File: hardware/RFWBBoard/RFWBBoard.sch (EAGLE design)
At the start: 123 parts, among them IC1 24LC025ST, J1 CON-71742-3003-BOT, M1 MOUNT-HOLE3.3, M2 MOUNT-HOLE3.3, M3 MOUNT-HOLE3.3, M4 MOUNT-HOLE3.3, M5 FIDUCIAL1X2, M6 FIDUCIAL1X2, M7 FIDUCIAL1X2, M8 FIDUCIAL1X2, U1 MAX2830IPC-7351, U2 LDB212G4010C-001, U3 LDB212G4010C-001, U4 AD8132MSOP8, U5 AD8132MSOP8, U6 AD8132MSOP8, U7 AD8132MSOP8, U8 ICS83021I, U9 ICS85320I, X1 SMA-SMD, X2 SMA-SMD, X3 FOX924B, X4 SMA-SMD, X5 SMA-SMD, X6 SMA-SMD, X7 SMA-SMD

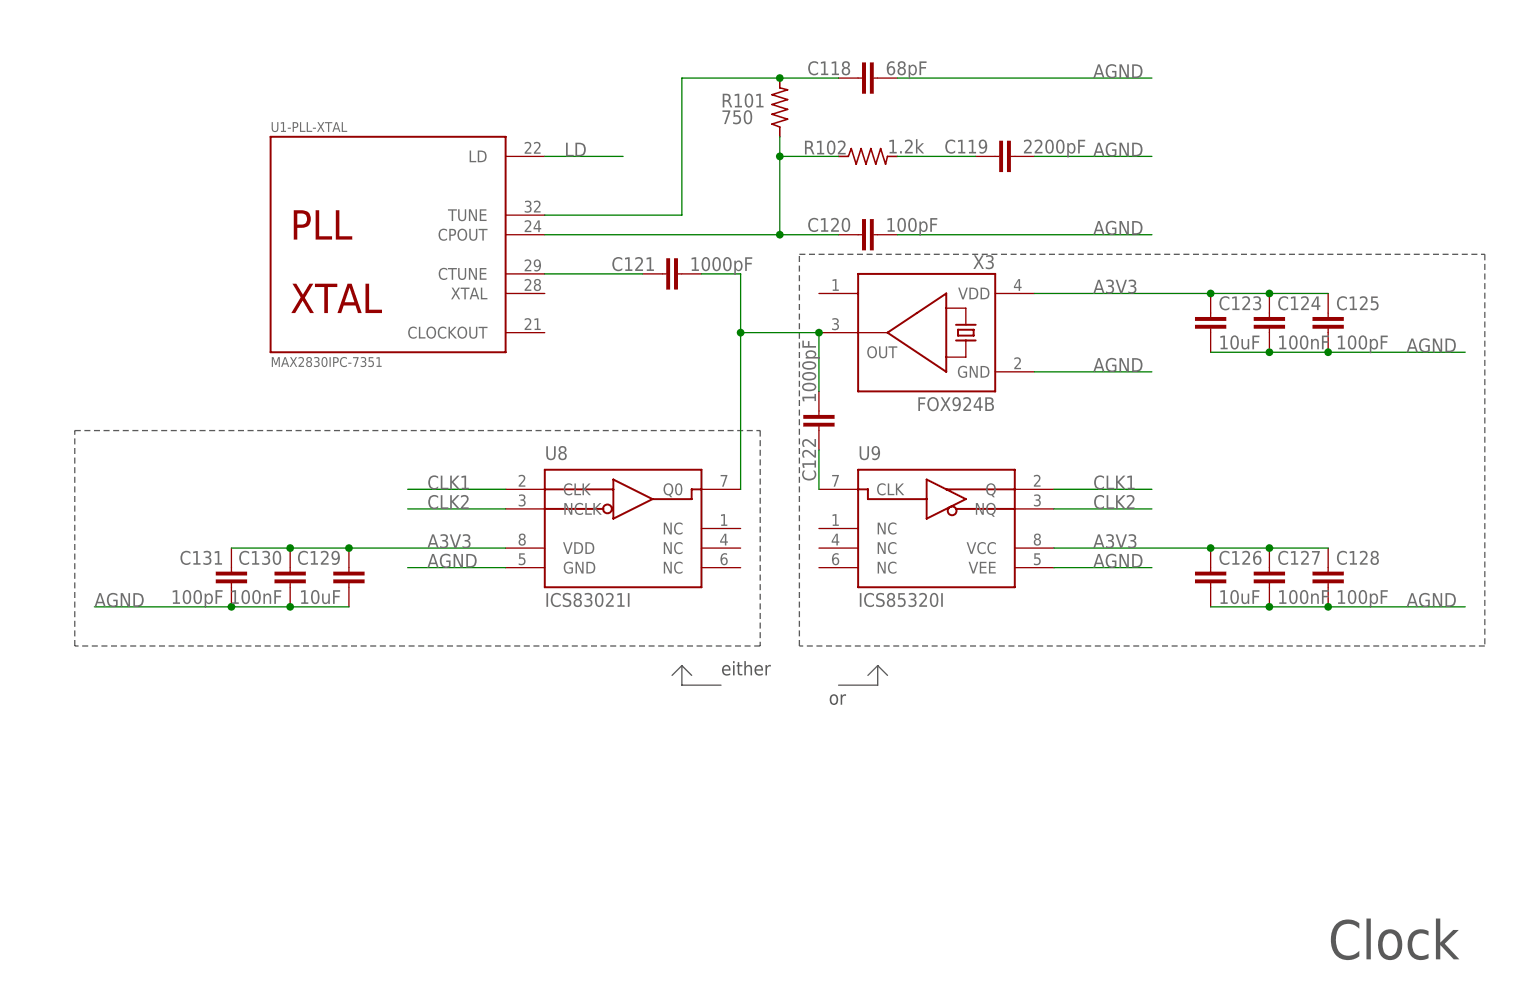
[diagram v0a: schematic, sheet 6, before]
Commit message: - Layout updated
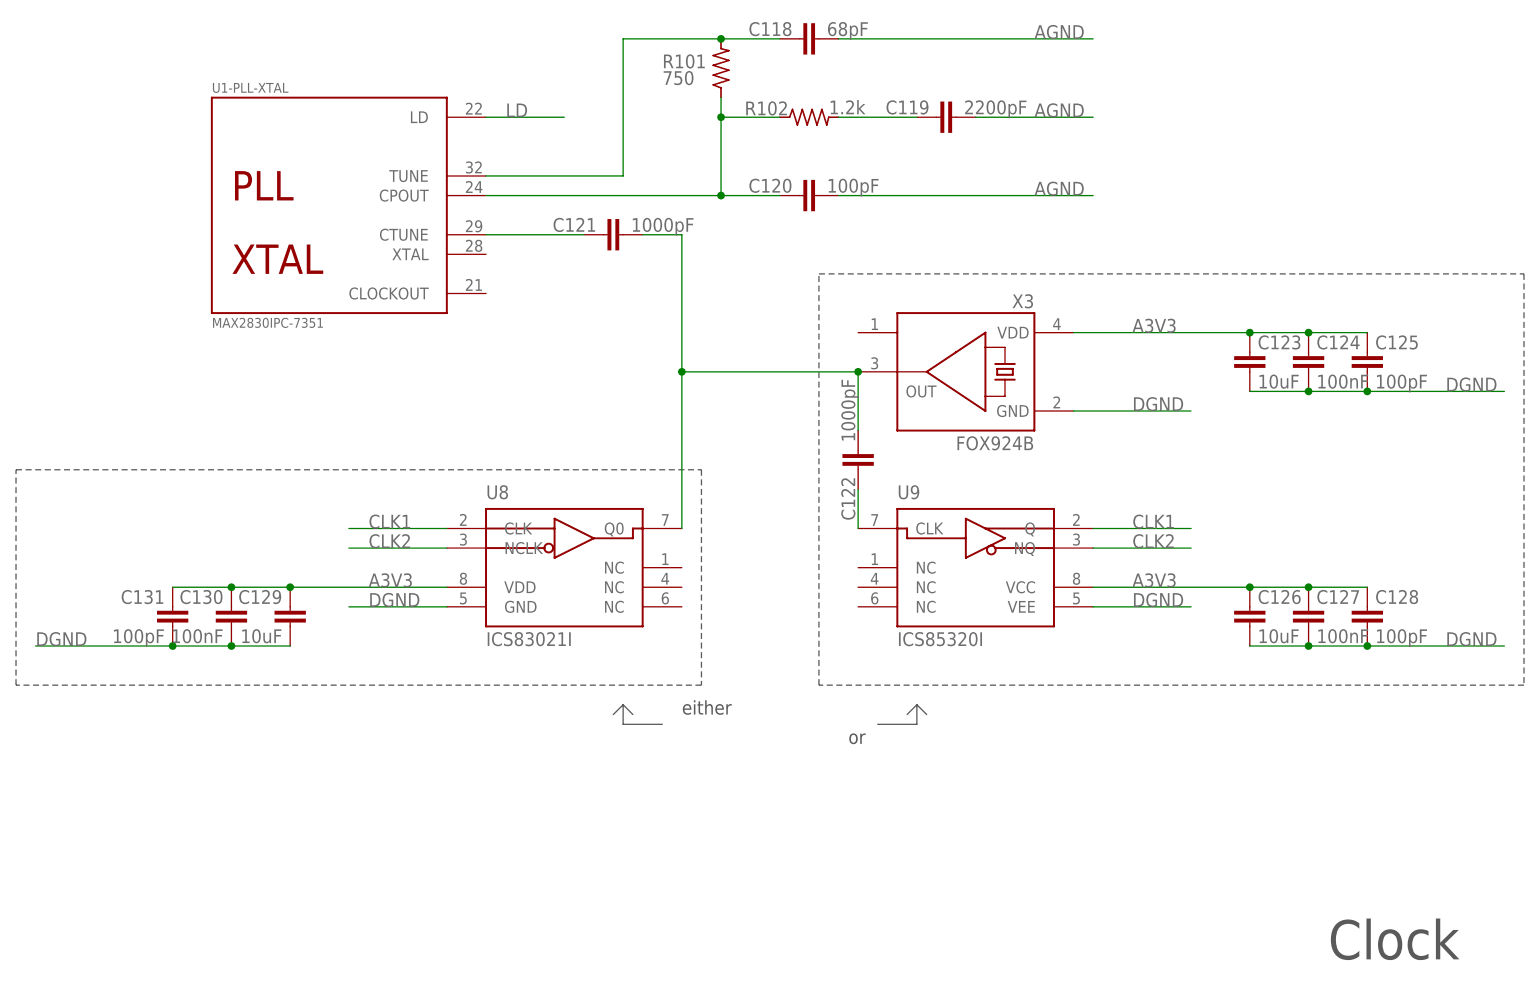
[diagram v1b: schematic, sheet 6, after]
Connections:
- net AGND: no longer C123.2, C124.2, C125.2, C126.2, C127.2, C128.2, C129.2, C130.2, C131.2, U8.GND, U9.VEE, X3.GND
- net DGND: now also C123.2, C124.2, C125.2, C126.2, C127.2, C128.2, C129.2, C130.2, C131.2, U8.GND, U9.VEE, X3.GND
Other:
- moved on the sheet: C118, C119, C120, C121, C122, C123, C124, C125, C126, C127, C128, C129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
